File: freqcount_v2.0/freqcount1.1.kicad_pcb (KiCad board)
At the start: 2 copper layers, 49.8 x 29.8 mm, 24 parts, among them J1 Conn_01x03_Male, J2 Conn_01x03_Male, J3 Conn_02x10_Odd_Even, J4 Conn_Coaxial, U1 74LS390, U10 MCP23017_SS, U2 74LS390, U3 74LS390, U4 74LS390, U5 74AHC1G04, U6 74LV8154, U7 MCP23017_SS, U8 74AHC1G04, U9 74LV8154

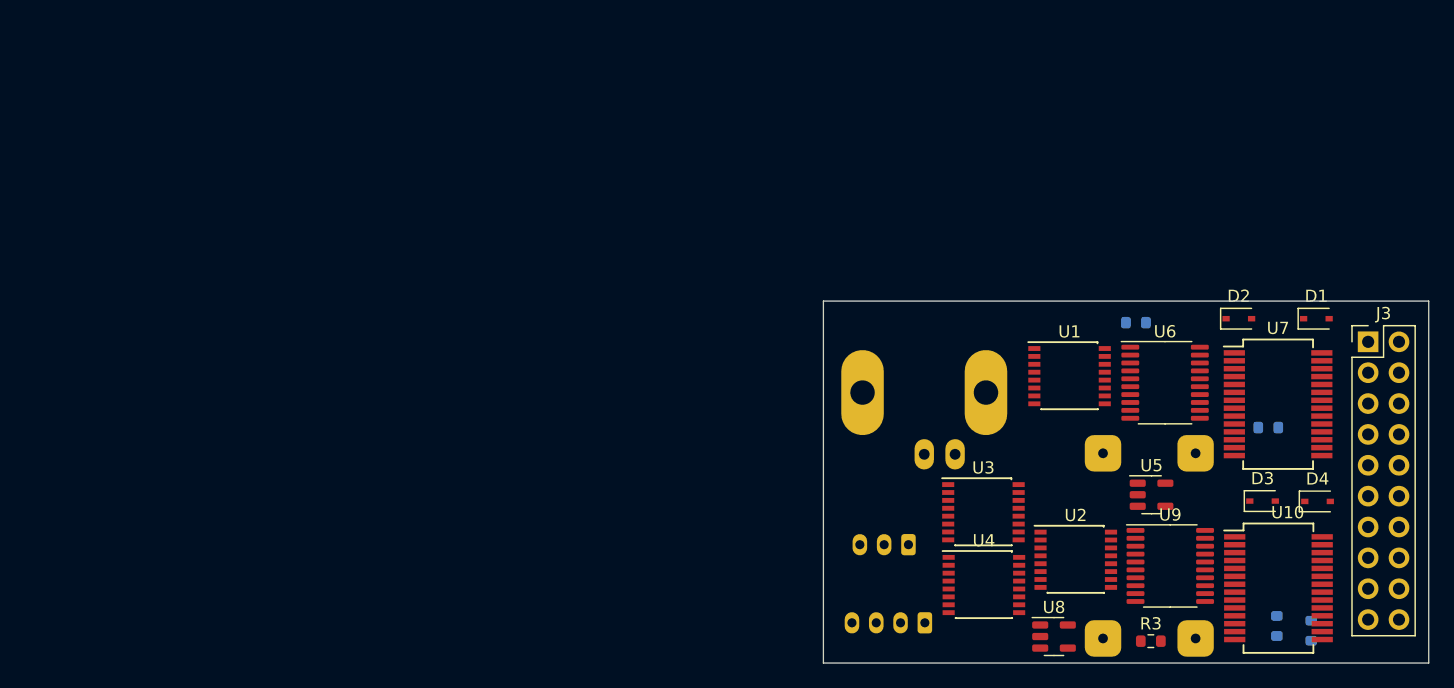
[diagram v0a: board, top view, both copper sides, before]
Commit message: update
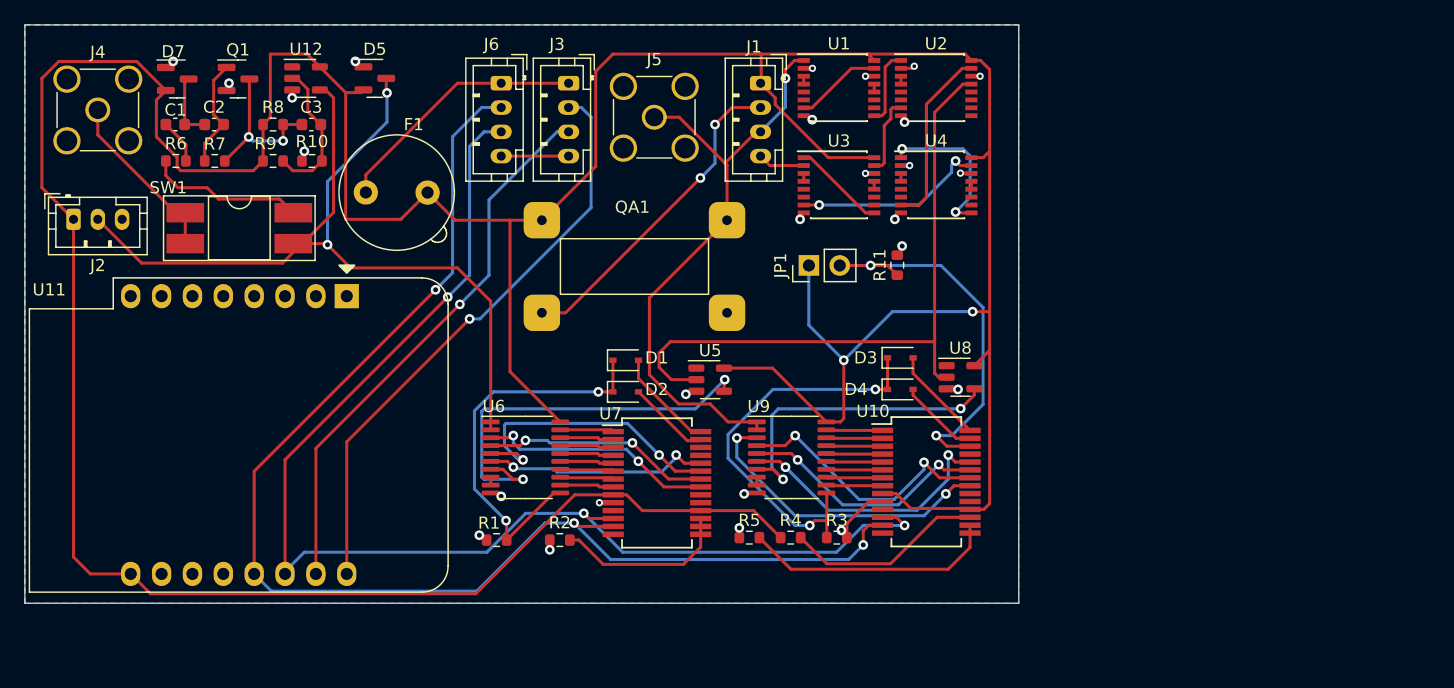
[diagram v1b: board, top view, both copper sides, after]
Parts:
- added C1: 100nF, Capacitor_SMD:C_0603_1608Metric, F.Cu at (51.6, 64.6)
- added C2: 100nF, Capacitor_SMD:C_0603_1608Metric, F.Cu at (54.8, 64.6)
- added C3: 100nF, Capacitor_SMD:C_0603_1608Metric, F.Cu at (62.8, 64.6)
- added D5: BAT54S, Package_TO_SOT_SMD:SOT-23, F.Cu at (68.0, 60.8)
- added D7: BAT54S, Package_TO_SOT_SMD:SOT-23, F.Cu at (51.7, 60.9)
- added F1: 500mA, Fuse:Fuseholder_TR5_Littelfuse_No560_No460, F.Cu at (67.3, 70.2)
- added J5: Conn_Coaxial, Connector_Coaxial:SMA_Amphenol_901-144_Vertical, F.Cu at (91.0, 64.0)
- added J6: Conn_01x04_Male, Connector_JST:JST_PH_B4B-PH-K_1x04_P2.00mm_Vertical, F.Cu at (78.4, 61.2)
- added JP1: Jumper_2_Open, Connector_PinHeader_2.54mm:PinHeader_1x02_P2.54mm_Vertical, F.Cu at (103.7, 76.2)
- added Q1: MMBT3904, Package_TO_SOT_SMD:SOT-23, F.Cu at (56.7, 60.9)
- added R10: 10k, Resistor_SMD:R_0603_1608Metric, F.Cu at (62.8, 67.6)
- added R11: 10k, Resistor_SMD:R_0603_1608Metric, F.Cu at (111.0, 76.2)
- added R6: 47R, Resistor_SMD:R_0603_1608Metric, F.Cu at (51.6, 67.6)
- added R7: 10k, Resistor_SMD:R_0603_1608Metric, F.Cu at (54.8, 67.6)
- added R8: 1k, Resistor_SMD:R_0603_1608Metric, F.Cu at (59.6, 64.6)
- added R9: 10k, Resistor_SMD:R_0603_1608Metric, F.Cu at (59.6, 67.6)
- added SW1: SW_DIP_x02, Package_DIP:DIP-4_W8.89mm_SMDSocket_LongPads, F.Cu at (56.8, 73.1)
- added U11: WeMos_D1_mini, Module:WEMOS_D1_mini_light, F.Cu at (65.7, 78.7)
- added U12: 74AHC1G04, Package_TO_SOT_SMD:SOT-23-5, F.Cu at (62.3, 60.8)
- J1, J2, QA1, R1, R2, R4, R5: moved to F.Cu
- J3: value Conn_02x10_Odd_Even -> Conn_01x04_Male; footprint Connector_PinHeader_2.54mm:PinHeader_2x10_P2.54mm_Vertical -> Connector_JST:JST_PH_B4B-PH-K_1x04_P2.00mm_Vertical
- J4: footprint Connector_Coaxial:BNC_Amphenol_B6252HB-NPP3G-50_Horizontal -> Connector_Coaxial:SMA_Amphenol_901-144_Vertical; moved to F.Cu
- moved J2 73.8 mm to (43.2, 72.4), turned to 0 degrees
- moved J4 73.7 mm to (45.2, 63.4), turned to 0 degrees
- moved J3 69.2 mm to (84.0, 61.2), turned to -90 degrees
- moved QA1 64.5 mm to (76.2, 85.2), turned to 0 degrees
- moved R2 59.0 mm to (83.2, 98.8), turned to 0 degrees
- moved D1 56.9 mm to (88.7, 84.0)
- moved R1 55.6 mm to (78.0, 98.8)
- moved U6 53.0 mm to (80.4, 92.0)
- moved U7 51.5 mm to (91.2, 94.1)
- moved D2 50.8 mm to (88.7, 86.6)
- moved J1 46.4 mm to (99.8, 61.2), turned to -90 degrees
- moved R5 44.0 mm to (98.8, 98.6), turned to 0 degrees
- moved R4 43.5 mm to (102.2, 98.6), turned to 0 degrees
- moved U2 40.5 mm to (114.2, 61.6)
- moved U5 37.5 mm to (95.6, 85.6)
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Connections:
- J2 pad 2: Net-(J2-Pad2) -> /Zaehler_Messsignal/Messsignal
- J3 pad 1: +5V -> Net-(F1-Pad1)
- J3 pad 3: GND -> Rx
- J3 pad 4: Rx -> GND
- J4 pad 1: Net-(J2-Pad2) -> Net-(J4-Pad1)
- U10 pad 26: unconnected-(U10-Pad26) -> /Zaehler_Referenz/measure_select
- U6 pad 1: Net-(J2-Pad2) -> /Zaehler_Messsignal/Messsignal
- U6 pad 2: Net-(J2-Pad2) -> /Zaehler_Messsignal/Messsignal
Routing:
- net +5V: track 0.00 -> 347.3 mm, vias 0 -> 2
- net /ESP/SDA: track 0.00 -> 108.8 mm, vias 0 -> 3
- net /ESP/SCK: track 0.00 -> 104.7 mm, vias 0 -> 3
- net /Zaehler_Messsignal/Messsignal: track 0.00 -> 78.4 mm, vias 0 -> 2
- net /Teiler_1Hz/1Hz_Puls: track 0.00 -> 54.3 mm
- net /Teiler_1Hz/10MHz_Referenz: track 0.00 -> 50.4 mm, vias 0 -> 1
- net Tx: track 0.00 -> 48.6 mm, vias 0 -> 1
- net Rx: track 0.00 -> 45.6 mm, vias 0 -> 1
- net Net-(U5-Pad4): track 0.00 -> 33.9 mm, vias 0 -> 2
- net Net-(D3-Pad1): track 0.00 -> 33.9 mm, vias 0 -> 2
- net Net-(D1-Pad1): track 0.00 -> 32.4 mm, vias 0 -> 2
- net /Zaehler_Referenz/measure_select: track 0.00 -> 31.8 mm, vias 0 -> 2
- net Net-(J1-Pad2): track 0.00 -> 26.9 mm, vias 0 -> 2
- net Net-(U8-Pad4): track 0.00 -> 26.0 mm, vias 0 -> 2
- net GAL2: track 0.00 -> 25.5 mm, vias 0 -> 2
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- added copper zone on B.Cu, net GND
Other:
- board size 49.8 x 29.8 mm -> 81.8 x 47.6 mm
